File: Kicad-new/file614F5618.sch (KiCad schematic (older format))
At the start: 109 parts, among them J1 V12, J10 I2C, J11 ILI9341, J12 Link-out 2-2, J13 Encoders, J2 Link-out 1-0, J3 Link-out 1-1, J4 Jtag, J5 Link-out 1-2, J6 Link-out 2-0, J7 Link-out 2-1, J8 I2C, J9 Analog in 3-6, Q1 BFR92, Q2 BFR92, Q3 BFR92, Q4 BFR92, Q5 BFR92, Q6 BFR92, Q7 2n3904, Q8 2N3904, SW1 Rotary_Encoder_Switch, U1 LM1117-3.3, U2 LM2576HVS-ADJ, U3 Si5351A-B-GT, U4 TCA9548APWR, U5 ESP32-WROOM-32D, U6 Si5351A-B-GT, Y1 Crystal, Y2 Crystal

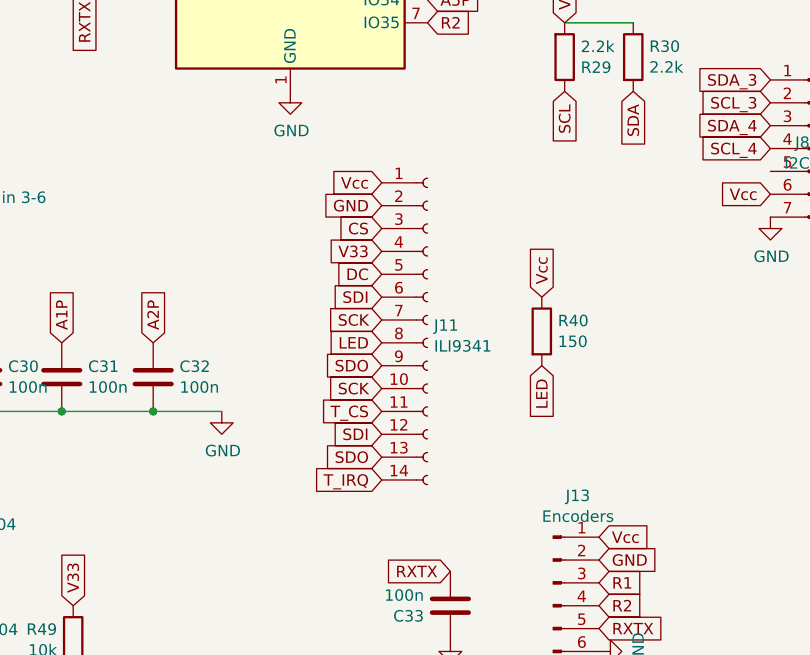
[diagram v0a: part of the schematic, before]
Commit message: new pcb
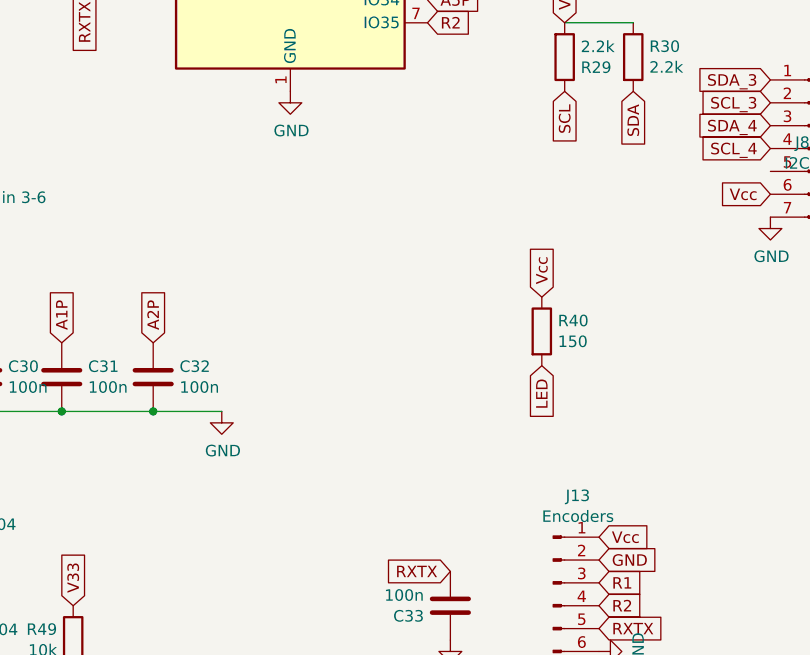
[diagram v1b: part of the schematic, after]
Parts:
- removed J11: ILI9341, Connector_PinSocket_2.54mm:PinSocket_1x14_P2.54mm_Vertical, symbol Connector:Conn_01x14_Female
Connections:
- net labels removed: T_IRQ
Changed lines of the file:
@@
 $Descr A4 11693 8268
 encoding utf-8
-Sheet 1 2
+Sheet 3 5
 Title ""
 Date ""
@@
 Comment4 ""
 $EndDescr
-$Comp
-L Connector:Conn_01x14_Female J11
-U 1 1 5D7C3C46
-P 3450 6000
-F 0 "J11" H 3478 5976 50  0000 L CNN
-F 1 "ILI9341" H 3478 5885 50  0000 L CNN
-F 2 "Connector_PinSocket_2.54mm:PinSocket_1x14_P2.54mm_Vertical" H 3450 6000 50  0001 C CNN
-F 3 "~" H 3450 6000 50  0001 C CNN
-	1    3450 6000
-	1    0    0    -1
-$EndComp
 Text GLabel 8700 800  1    50   Input ~ 0
 V33
 Text GLabel 8300 2250 0    50   Input ~ 0
 SDA_1
-Text GLabel 3250 5400 0    50   Input ~ 0
-Vcc
-Text GLabel 3250 5500 0    50   Input ~ 0
-GND
-Text GLabel 3250 5600 0    50   Input ~ 0
-CS
-Text GLabel 3250 5800 0    50   Input ~ 0
-DC
-Text GLabel 3250 5900 0    50   Input ~ 0
-SDI
-Text GLabel 3250 6000 0    50   Input ~ 0
-SCK
-Text GLabel 3250 6100 0    50   Input ~ 0
-LED
-Text GLabel 3250 6200 0    50   Input ~ 0
-SDO
-Text GLabel 3250 6400 0    50   Input ~ 0
-T_CS
-Text GLabel 3250 6700 0    50   Input ~ 0
-T_IRQ
 Text GLabel 3450 2600 2    50   Input ~ 0
 DC
@@
 Text GLabel 1100 5200 0    50   Input ~ 0
 A1P
-Text GLabel 3250 6300 0    50   Input ~ 0
-SCK
-Text GLabel 3250 6500 0    50   Input ~ 0
-SDI
-Text GLabel 3250 5700 0    50   Input ~ 0
-V33
 Text GLabel 3450 4300 2    50   Input ~ 0
 SDO
-Text GLabel 3250 6600 0    50   Input ~ 0
-SDO
 Wire Wire Line
